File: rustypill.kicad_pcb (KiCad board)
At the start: 2 copper layers, 69 x 45.5 mm, 48 parts, among them IC1 DS3231, J1 USB, J2 PROG, J3 GPIOB, J4 GPIOA, J5 LCD1602, J6 IDC_10P, M2 MountingHole_2.7mm_M2.5, M3 MountingHole_2.7mm_M2.5, M4 MountingHole_2.7mm_M2.5, U1 AMS1117-3.3, U2 AT24C512C-SSHD-T, U3 ESP-12F, U4 STM32F103C8Tx, Y1 8MHz

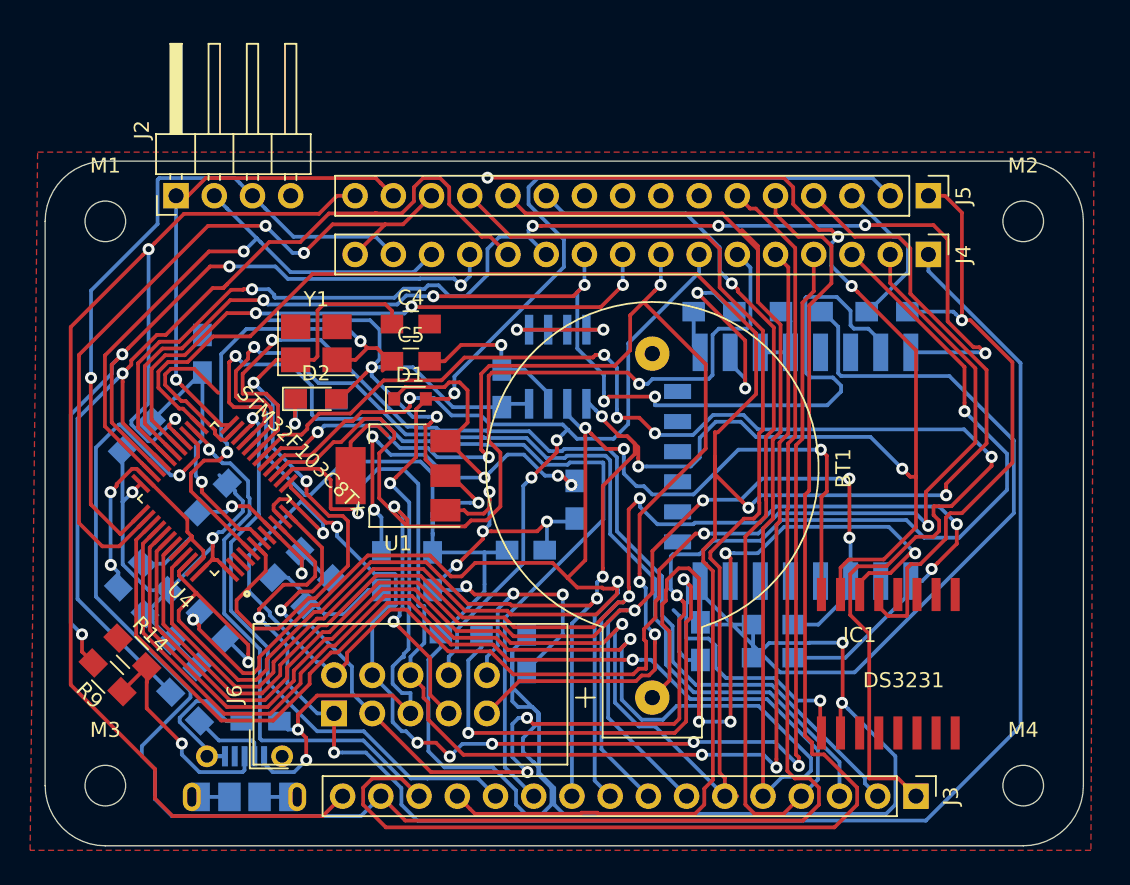
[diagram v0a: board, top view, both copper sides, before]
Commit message: ...
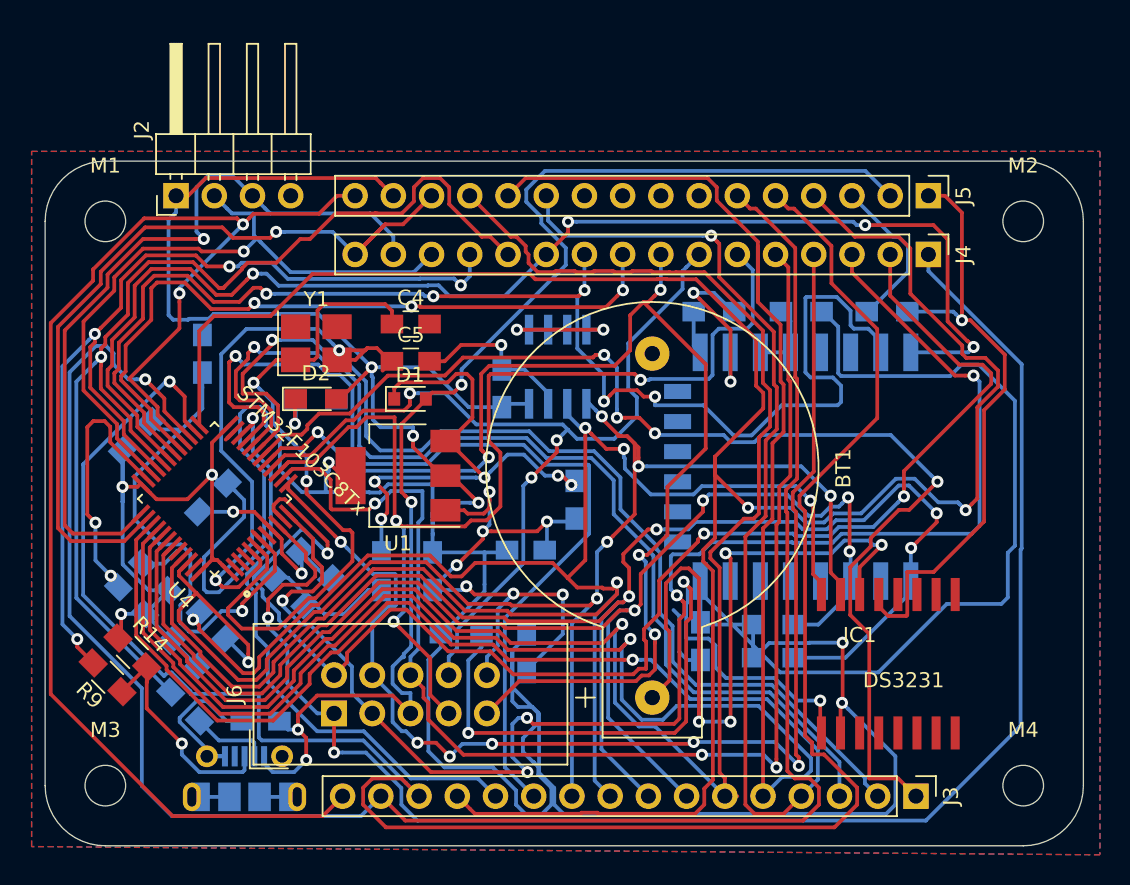
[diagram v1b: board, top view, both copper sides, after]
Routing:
- net B9: track 157.3 -> 100.4 mm, vias 9 -> 6
- net +3V3: track 298.4 -> 331.4 mm, vias 8 -> 9
- net Net-(C6-Pad1): track 18.4 -> 35.1 mm
- net B13: track 121.3 -> 137.8 mm
- net GND: track 170.7 -> 157.2 mm
- net B0: track 89.5 -> 80.3 mm
- net A9: track 81.4 -> 90.1 mm
- net A8: track 41.6 -> 48.3 mm
- net A11: track 66.7 -> 73.1 mm
- net A12: track 59.4 -> 65.3 mm
- net Net-(C5-Pad1): track 32.8 -> 38.1 mm
- net A14: track 45.9 -> 51.0 mm
- net Net-(BT1-Pad1): track 53.6 -> 48.8 mm
- net A13: track 39.4 -> 44.3 mm
- net B8: track 136.7 -> 131.9 mm
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- added copper zone on B.Cu, net GND

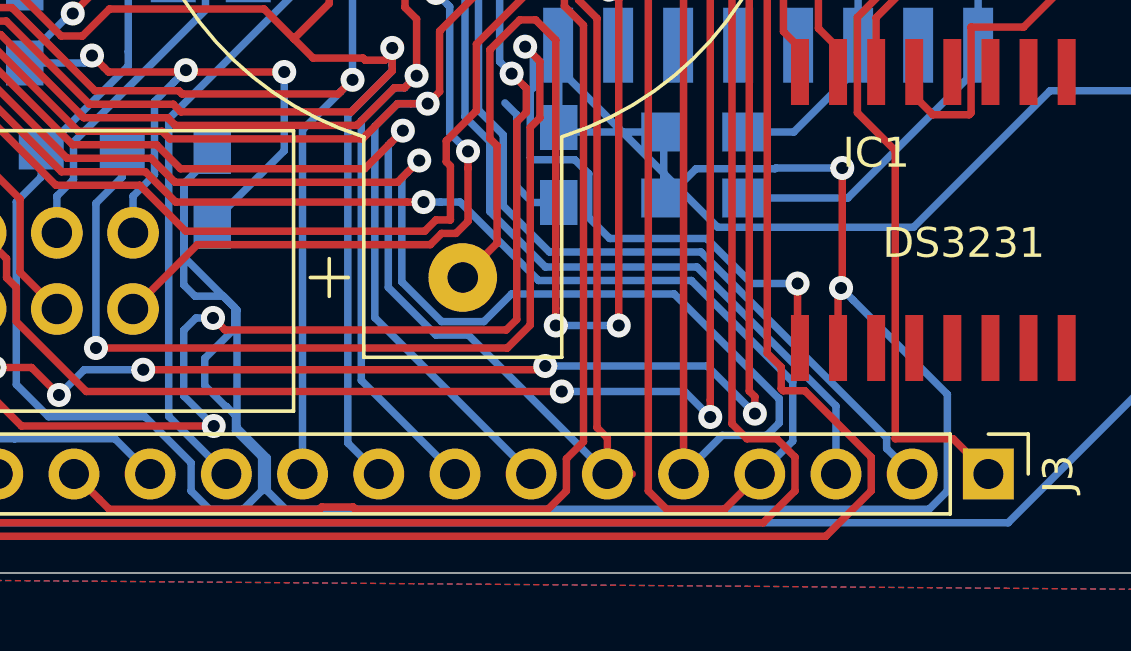
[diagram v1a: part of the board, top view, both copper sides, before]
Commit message: ...
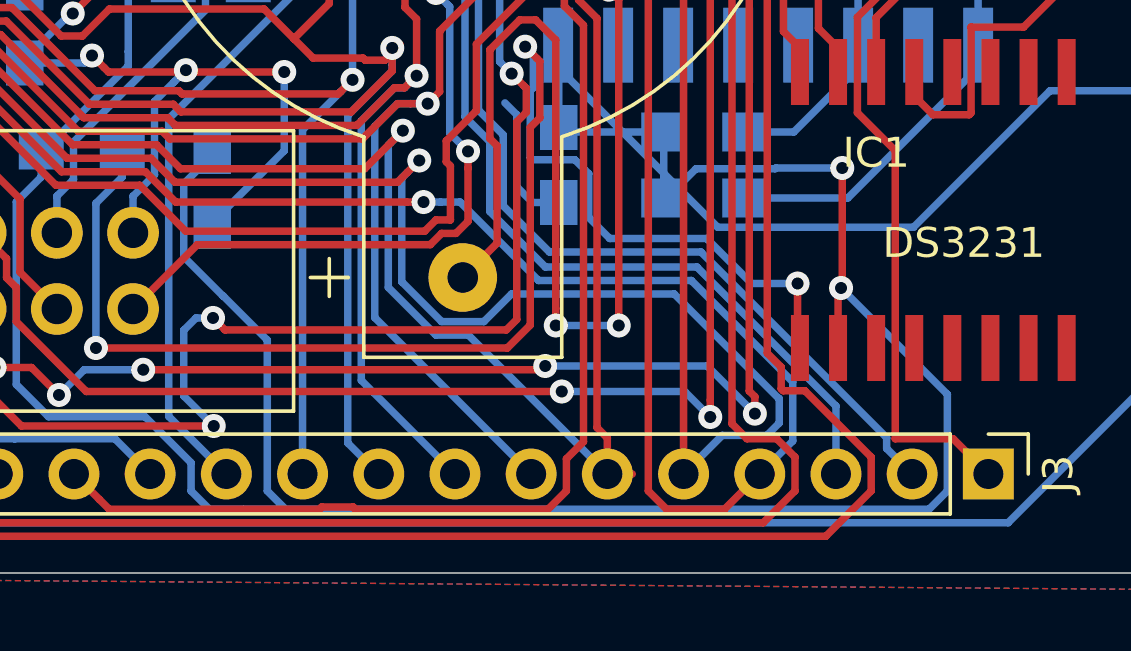
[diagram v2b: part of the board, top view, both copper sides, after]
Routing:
- net +3V3: track 331.4 -> 319.3 mm
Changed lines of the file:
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@@
     (thickness 1.6)
     (drawings 8)
-    (tracks 1914)
+    (tracks 1900)
     (zones 0)
     (modules 48)
@@
   (segment (start 99.294999 137.264001) (end 99.905999 137.875001) (width 0.25) (layer B.Cu) (net 4))
   (segment (start 99.905999 137.875001) (end 101.034001 137.875001) (width 0.25) (layer B.Cu) (net 4))
-  (segment (start 101.034001 137.875001) (end 101.645001 137.264001) (width 0.25) (layer B.Cu) (net 4))
-  (segment (start 101.645001 137.264001) (end 101.645001 136.135999) (width 0.25) (layer B.Cu) (net 4))
-  (segment (start 100.775001 134.751999) (end 100.47501 134.452008) (width 0.25) (layer B.Cu) (net 4))
-  (segment (start 101.645001 136.135999) (end 100.775001 135.265999) (width 0.25) (layer B.Cu) (net 4))
-  (segment (start 100.775001 135.265999) (end 100.775001 134.751999) (width 0.25) (layer B.Cu) (net 4))
-  (segment (start 100.47501 134.452008) (end 100.452008 134.452008) (width 0.25) (layer B.Cu) (net 4))
-  (segment (start 100.452008 134.452008) (end 99.75 133.75) (width 0.25) (layer B.Cu) (net 4))
-  (segment (start 100.75 131.150179) (end 100.373001 130.77318) (width 0.25) (layer B.Cu) (net 4))
-  (segment (start 100.373001 130.77318) (end 99.42682 130.77318) (width 0.25) (layer B.Cu) (net 4))
-  (segment (start 100.75 131.846183) (end 100.75 131.150179) (width 0.25) (layer B.Cu) (net 4))
-  (segment (start 99.75 133.75) (end 99.75 132.846183) (width 0.25) (layer B.Cu) (net 4))
-  (segment (start 99.75 132.846183) (end 100.75 131.846183) (width 0.25) (layer B.Cu) (net 4))
-  (segment (start 99.049999 127.025001) (end 100 126.075) (width 0.25) (layer B.Cu) (net 4))
-  (segment (start 100 126.075) (end 100 125.95) (width 0.25) (layer B.Cu) (net 4))
-  (segment (start 99.049999 130.396359) (end 99.049999 127.025001) (width 0.25) (layer B.Cu) (net 4))
-  (segment (start 99.42682 130.77318) (end 99.049999 130.396359) (width 0.25) (layer B.Cu) (net 4))
   (segment (start 115.05 127.5) (end 115.05 125.3) (width 0.25) (layer B.Cu) (net 4))
   (segment (start 111.7 125.3) (end 111.55 125.15) (width 0.25) (layer B.Cu) (net 4))
@@
   (segment (start 121 126.5) (end 118.785 126.5) (width 0.25) (layer B.Cu) (net 4))
   (segment (start 93.75 120.5) (end 93.75 120.375) (width 0.25) (layer B.Cu) (net 4))
-  (segment (start 101.834999 137.264001) (end 102.445999 137.875001) (width 0.25) (layer B.Cu) (net 4))
-  (segment (start 121.360009 130.899999) (end 120.96001 130.5) (width 0.25) (layer B.Cu) (net 4))
-  (segment (start 124.505001 137.264001) (end 124.505001 134.044991) (width 0.25) (layer B.Cu) (net 4))
   (segment (start 120.86 132.5) (end 120.86 130.60001) (width 0.25) (layer F.Cu) (net 4))
-  (segment (start 99.049999 127.025001) (end 99.049999 129.460001) (width 0.25) (layer B.Cu) (net 4))
   (segment (start 121 126.5) (end 121 130.46001) (width 0.25) (layer F.Cu) (net 4))
   (segment (start 120.86 130.60001) (end 120.96001 130.5) (width 0.25) (layer F.Cu) (net 4))
-  (segment (start 101.834999 136.161409) (end 101.834999 137.264001) (width 0.25) (layer B.Cu) (net 4))
-  (segment (start 123.894001 137.875001) (end 124.505001 137.264001) (width 0.25) (layer B.Cu) (net 4))
   (segment (start 121 130.46001) (end 120.96001 130.5) (width 0.25) (layer F.Cu) (net 4))
-  (segment (start 100.82499 131.234992) (end 100.82499 135.1514) (width 0.25) (layer B.Cu) (net 4))
-  (segment (start 99.049999 129.460001) (end 100.82499 131.234992) (width 0.25) (layer B.Cu) (net 4))
   (via (at 120.96001 130.5) (size 0.8) (drill 0.4) (layers F.Cu B.Cu) (net 4))
-  (segment (start 100.82499 135.1514) (end 101.834999 136.161409) (width 0.25) (layer B.Cu) (net 4))
-  (segment (start 102.445999 137.875001) (end 123.894001 137.875001) (width 0.25) (layer B.Cu) (net 4))
-  (segment (start 124.505001 134.044991) (end 121.360009 130.899999) (width 0.25) (layer B.Cu) (net 4))
   (segment (start 94.3 125.9) (end 94.4 125.9) (width 0.25) (layer B.Cu) (net 4))
   (segment (start 97.2 123.1) (end 97.2 122.623002) (width 0.25) (layer B.Cu) (net 4))
@@
   (segment (start 89.699998 108.2) (end 86.149998 104.65) (width 0.25) (layer B.Cu) (net 4))
   (segment (start 86.149998 104.65) (end 79.2 104.65) (width 0.25) (layer B.Cu) (net 4))
+  (segment (start 120.96001 130.5) (end 124.505001 134.044991) (width 0.25) (layer B.Cu) (net 4))
+  (segment (start 124.505001 137.264001) (end 123.894001 137.875001) (width 0.25) (layer B.Cu) (net 4))
+  (segment (start 124.505001 134.044991) (end 124.505001 137.264001) (width 0.25) (layer B.Cu) (net 4))
+  (segment (start 123.894001 137.875001) (end 102.445999 137.875001) (width 0.25) (layer B.Cu) (net 4))
+  (segment (start 101.034001 137.875001) (end 102.445999 137.875001) (width 0.25) (layer B.Cu) (net 4))
+  (segment (start 99.049999 127.025001) (end 100 126.075) (width 0.25) (layer B.Cu) (net 4))
+  (segment (start 99.049999 129.460001) (end 99.049999 127.025001) (width 0.25) (layer B.Cu) (net 4))
+  (segment (start 101.834999 137.264001) (end 101.834999 132.235178) (width 0.25) (layer B.Cu) (net 4))
+  (segment (start 102.445999 137.875001) (end 101.834999 137.264001) (width 0.25) (layer B.Cu) (net 4))
+  (segment (start 101.834999 132.235178) (end 100.373001 130.77318) (width 0.25) (layer B.Cu) (net 4))
+  (segment (start 100.373001 130.77318) (end 100.363178 130.77318) (width 0.25) (layer B.Cu) (net 4))
+  (segment (start 100 126.075) (end 100 125.95) (width 0.25) (layer B.Cu) (net 4))
+  (segment (start 100.363178 130.77318) (end 99.049999 129.460001) (width 0.25) (layer B.Cu) (net 4))
   (segment (start 91.05 104.45) (end 91.05 105.325) (width 0.25) (layer F.Cu) (net 5))
   (segment (start 90.599986 103.999986) (end 91.05 104.45) (width 0.25) (layer F.Cu) (net 5))

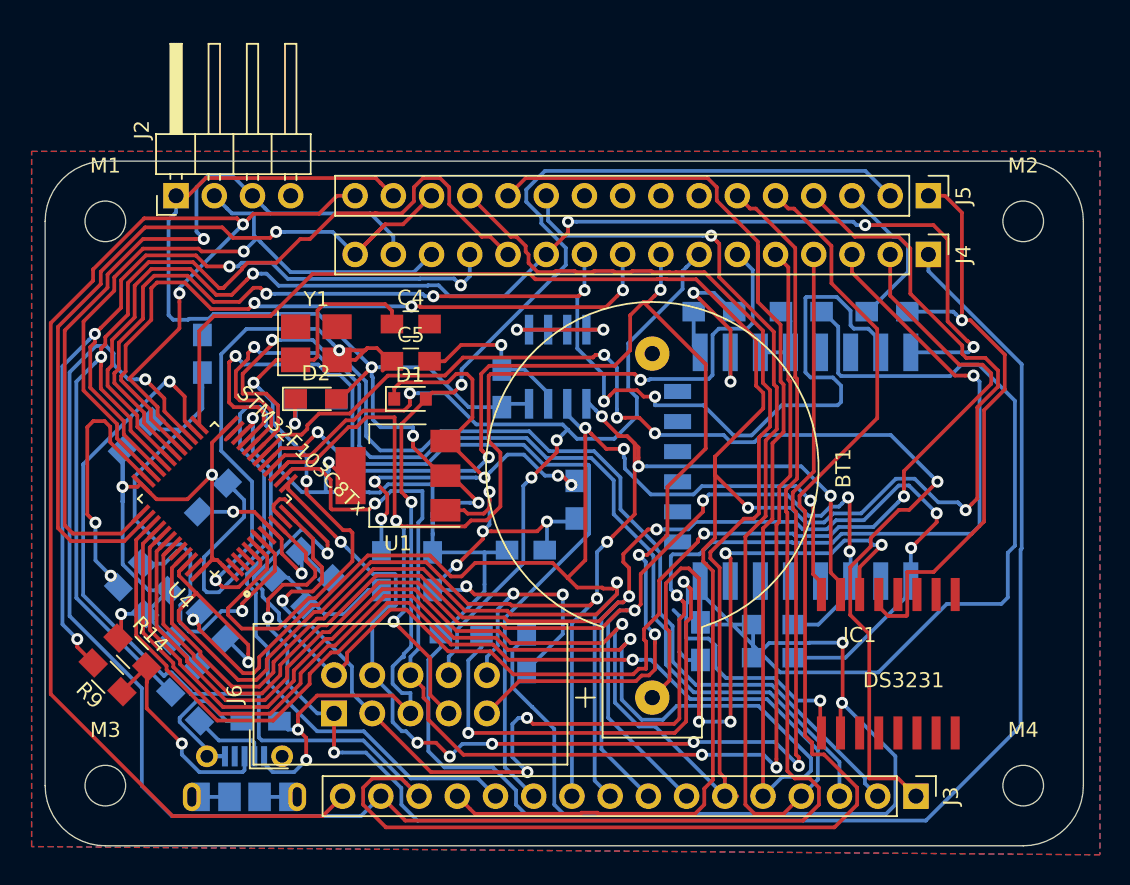
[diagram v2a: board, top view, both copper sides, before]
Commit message: ...
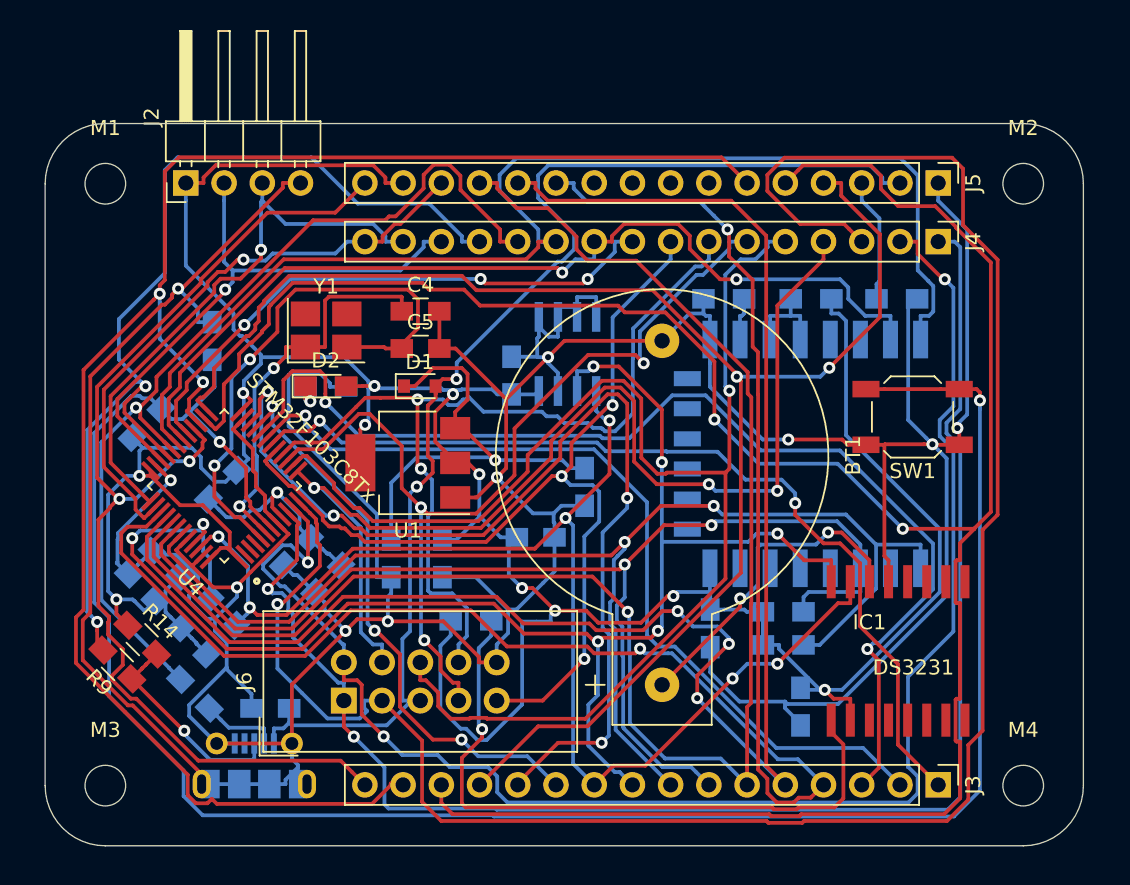
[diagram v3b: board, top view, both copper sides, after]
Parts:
- added SW1: Reset, Buttons_Switches_SMD:SW_SPST_SKQG, F.Cu at (125.7, 111.5)
- moved C11 18.5 mm to (118.2, 130.8)
- moved  M1 2.50 mm to (72.0, 96.0)
- moved M2 2.50 mm to (133.0, 96.0)
- moved J3 1.66 mm to (127.3, 135.9)
- moved C8 1.07 mm to (86.8, 122.3)
- moved C15 1.07 mm to (83.0, 130.9)
- moved C10 1.07 mm to (74.4, 122.8)
- moved C13 1.07 mm to (112.2, 125.5)
- moved C4 1.07 mm to (93.0, 104.5)
- moved IC1 1.07 mm to (124.7, 127.0)
- moved R10 1.07 mm to (78.0, 124.5)
- moved R11 1.07 mm to (79.7, 126.3)
- moved R14 1.07 mm to (74.5, 126.3)
- moved J4 1.07 mm to (127.3, 99.8)
- moved R12 1.07 mm to (96.3, 125.0)
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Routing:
- net GND: track 157.2 -> 349.5 mm, vias 13 -> 10
- net Net-(C6-Pad1): track 35.1 -> 137.3 mm, vias 1 -> 2
- net +3V3: track 319.3 -> 220.9 mm, vias 9 -> 11
- net B12: track 147.7 -> 103.4 mm
- net A2: track 101.0 -> 134.1 mm, vias 5 -> 1
- net B8: track 131.9 -> 101.4 mm, vias 5 -> 7
- net B11: track 39.1 -> 68.3 mm, vias 1 -> 4
- net A9: track 90.1 -> 62.6 mm, vias 5 -> 2
- net Net-(BT1-Pad1): track 48.8 -> 21.9 mm, vias 4 -> 2
- net B10: track 63.5 -> 38.0 mm, vias 1 -> 3
- net B14: track 133.1 -> 111.9 mm, vias 1 -> 2
- net B13: track 137.8 -> 158.7 mm, vias 1 -> 2
- net Net-(C4-Pad1): track 45.7 -> 26.4 mm
- net B0: track 80.3 -> 61.4 mm, vias 4 -> 2
- net B15: track 91.5 -> 73.6 mm
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- removed copper zone on B.Cu, net GND
- removed copper zone on F.Cu, net GND
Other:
- board size 69 x 45.5 mm -> 69 x 48 mm
